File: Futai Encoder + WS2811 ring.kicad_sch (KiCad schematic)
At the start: 42 parts, among them J1 Conn_02x05_Top_Bottom, SW1 RotaryEncoder_Switch_RGB

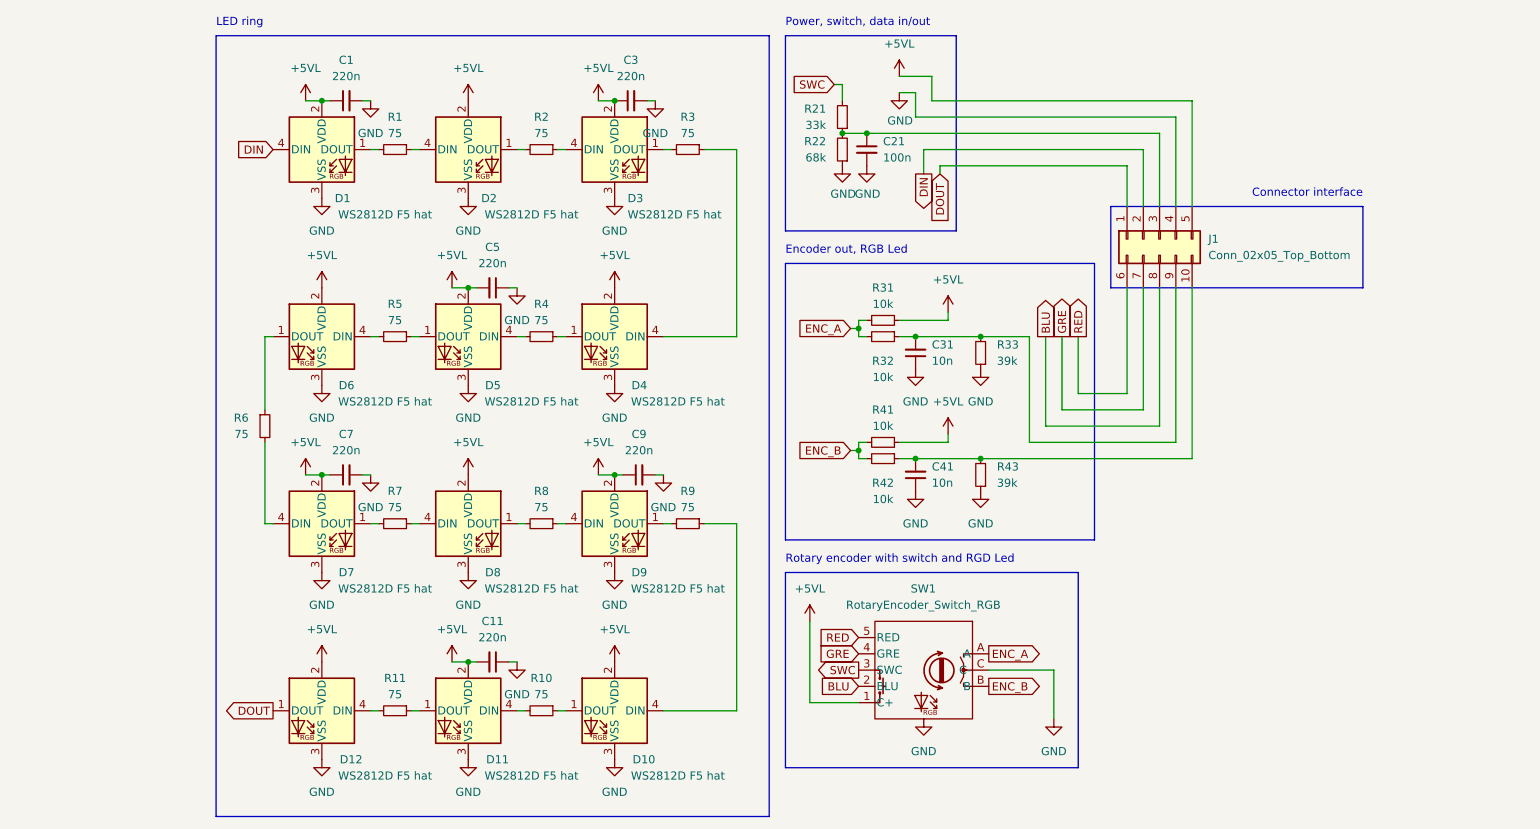
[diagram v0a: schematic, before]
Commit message: v0.9
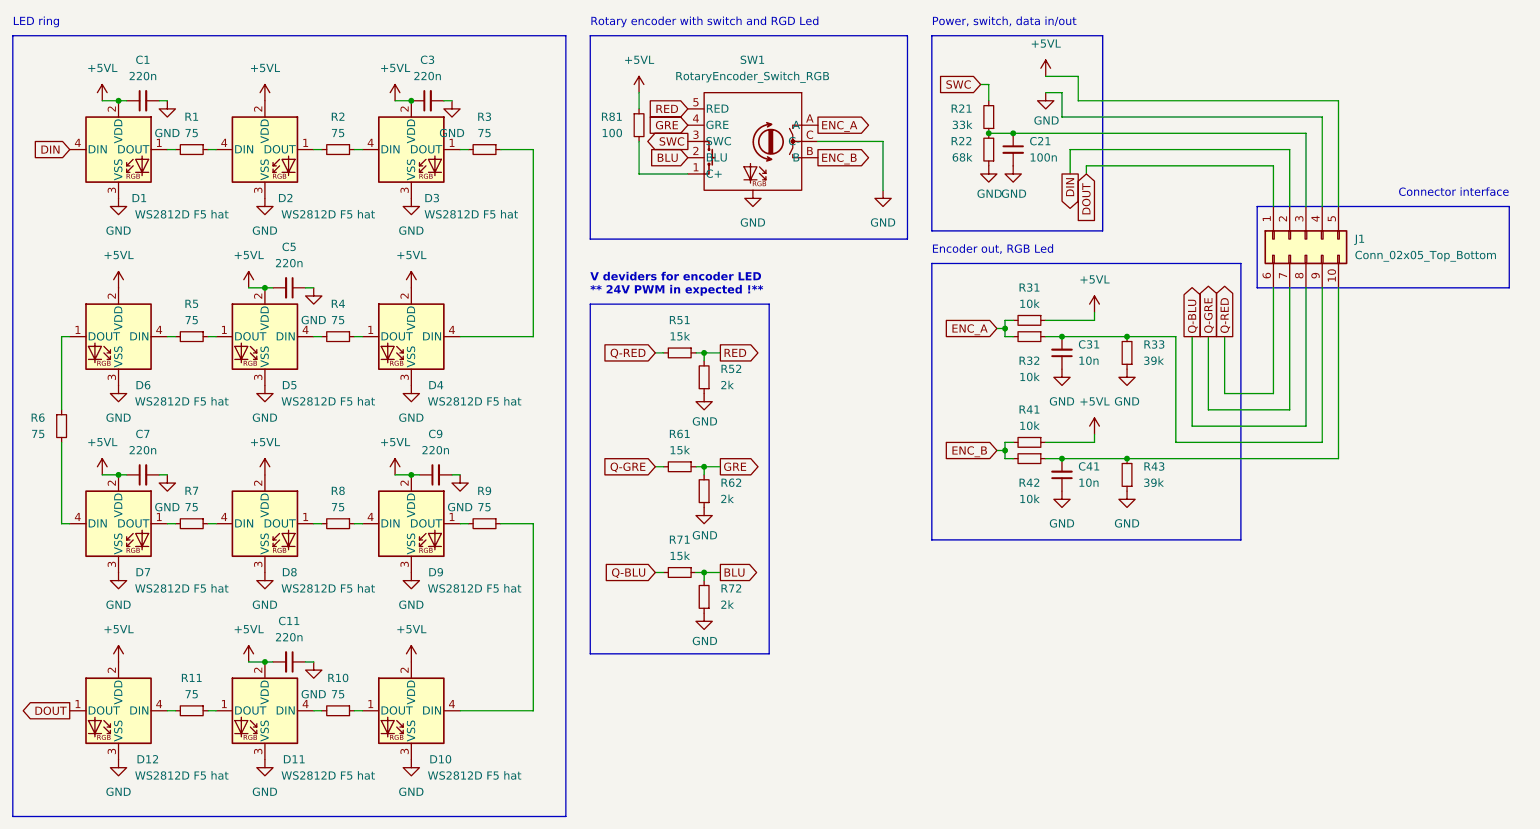
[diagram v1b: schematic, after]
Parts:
- added R51, R61, R71: 15k, Resistor_SMD:R_0805_2012Metric, symbol Device:R_Small
- added R52, R62, R72: 2k, Resistor_SMD:R_0805_2012Metric, symbol Device:R_Small
- added R81: 100, Resistor_SMD:R_0805_2012Metric, symbol Device:R_Small
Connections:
- net +5VL: now also R81.1; no longer SW1.1 (C+)
- net BLU: now also R71.1, R72.2; no longer J1.8 (Pin_8)
- net GND: now also R52.1, R62.1, R72.1
- net GRE: now also R61.1, R62.2; no longer J1.7 (Pin_7)
- net RED: now also R51.1, R52.2; no longer J1.6 (Pin_6)
- new net: R81.2, SW1.1 (C+)
- new net Q-BLU: J1.8 (Pin_8), R71.2
- new net Q-GRE: J1.7 (Pin_7), R61.2
- new net Q-RED: J1.6 (Pin_6), R51.2
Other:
- note added: "V deviders for encoder LED ** 24V PWM in expected !**"
- moved on the sheet: C1, C11, C21, C3, C31, C41, C5, C7, C9, D1, D10, D11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
